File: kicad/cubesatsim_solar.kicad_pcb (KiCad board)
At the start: 2 copper layers, 71.3 x 69.8 mm, 28 parts, among them J1 Sensor Inputs, J10 INA219 Sensor Board, J11 INA219 Sensor Board, J12 INA219 Sensor Board, J2 Battery In/Out, J3 Vdc In, J4 Vout to MoPOWER, J5 RBF Switch, J6 Expansion Interface, J7 INA219 Sensor Board, J8 INA219 Sensor Board, J9 INA219 Sensor Board

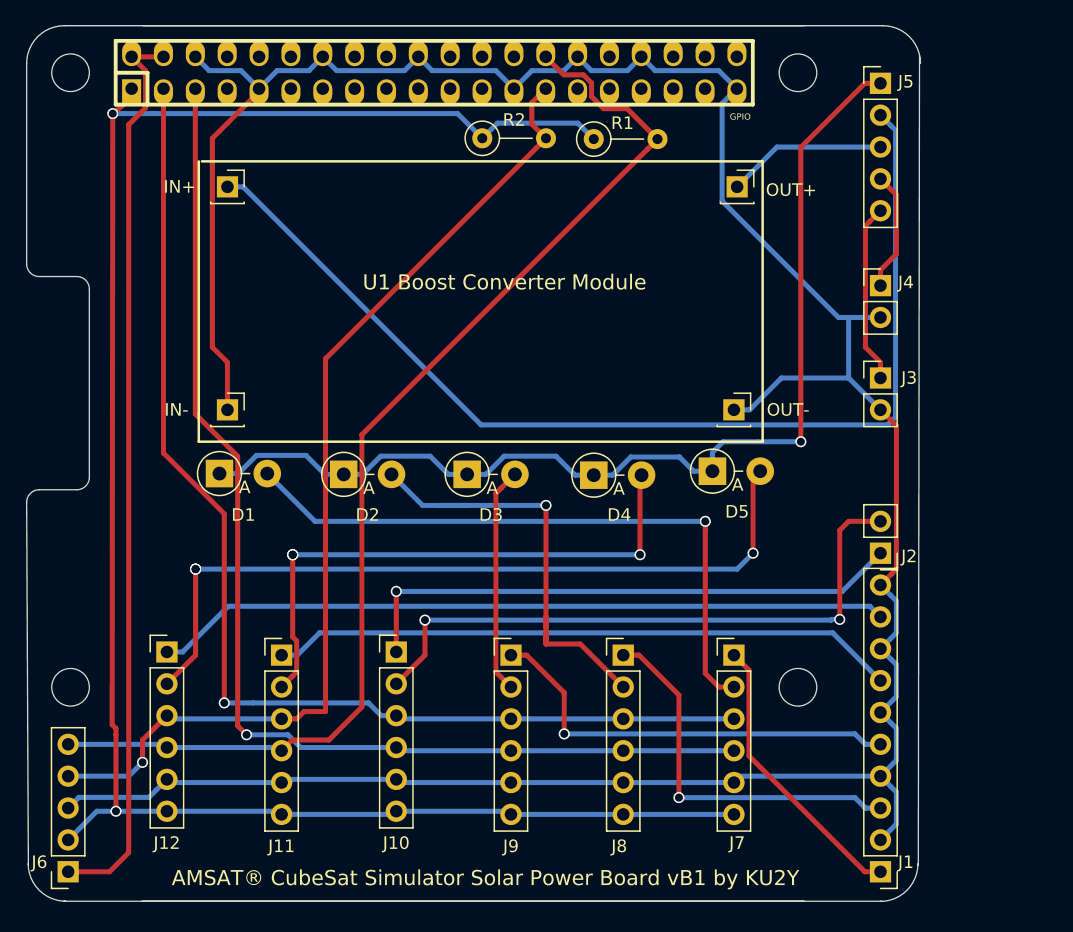
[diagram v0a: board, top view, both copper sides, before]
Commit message: vB2 PCB Submitted to PCB Way
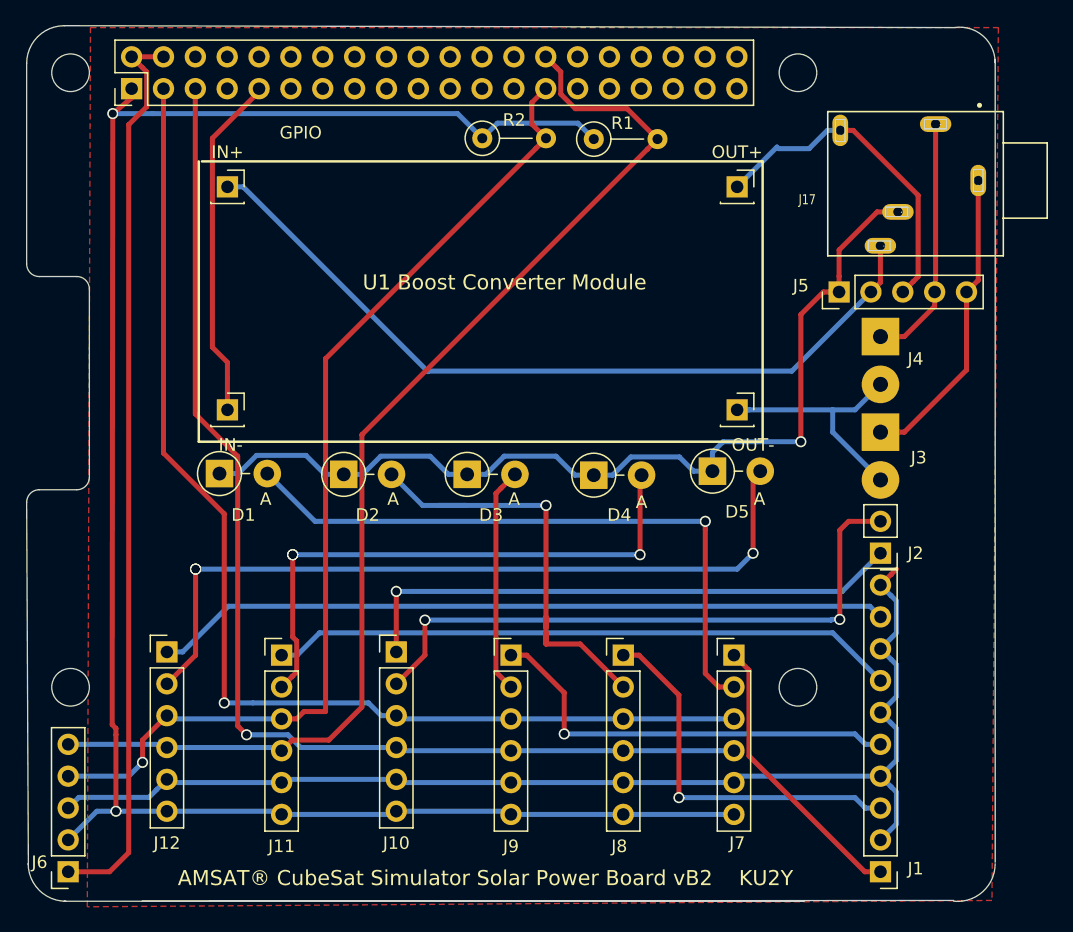
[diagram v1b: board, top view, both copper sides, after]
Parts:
- removed the GPIO at (137.4, 74.8)
- added GPIO: GPIO Male Extra Long (19mm) 20x2 Header Pins, Connector_PinHeader_2.54mm:PinHeader_2x20_P2.54mm_Vertical, F.Cu at (113.3, 76.1)
- added J17: , 35RAPC4BH3:SWITCHCRAFT_35RAPC4BH3, F.Cu at (175.8, 83.7)
- D1, D2, D3, D4, D5: value D -> 1N5817
- J3, J4: footprint Connector_PinHeader_2.54mm:PinHeader_1x02_P2.54mm_Vertical -> Connector_Wire:SolderWirePad_1x02_P3.81mm_Drill1.2mm
- moved J5 17.0 mm to (169.7, 92.3), turned to 90 degrees
- moved J3 4.32 mm to (173.0, 103.5), turned to 270 degrees
- moved J4 4.06 mm to (173.0, 95.9), turned to 270 degrees
- moved OUT- 0.25 mm to (161.6, 101.7)
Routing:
- net GND: track 228.2 -> 140.9 mm
- net Net-(J13-Pad1): track 86.0 -> 64.0 mm
- net Net-(J15-Pad1): track 12.7 -> 26.8 mm
- net Net-(J17-Pad1): track 14.3 -> 24.7 mm
- net Net-(J17-Pad5): track 9.56 -> 19.9 mm
- net Net-(D1-Pad1): track 84.9 -> 76.2 mm
- added copper zone on F.Cu, net GND
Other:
- board size 71.3 x 69.8 mm -> 77.2 x 69.8 mm
- board text added: "AMSAT® CubeSat Simulator Solar Power Board vB2 KU2Y"
- board text removed: "AMSAT® CubeSat Simulator Solar Power Board vB1 by KU2Y"
